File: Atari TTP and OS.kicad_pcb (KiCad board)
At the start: 2 copper layers, 19.6 x 52.1 mm, 13 parts, among them J1 Left, J2 Right, J4 Signals, J6 TTP_sel, U1 74LS157, U2 27C010, U3 74LVC2G74

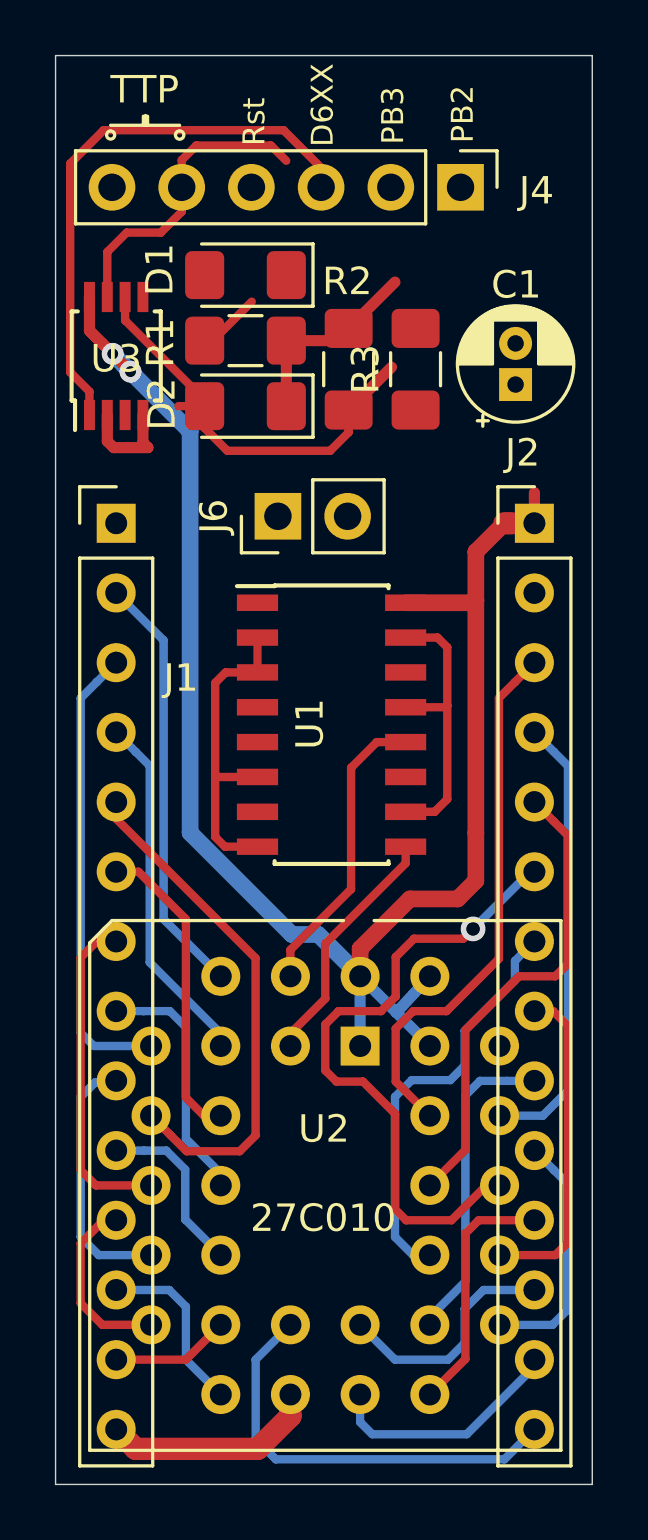
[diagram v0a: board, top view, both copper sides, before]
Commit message: Tracking
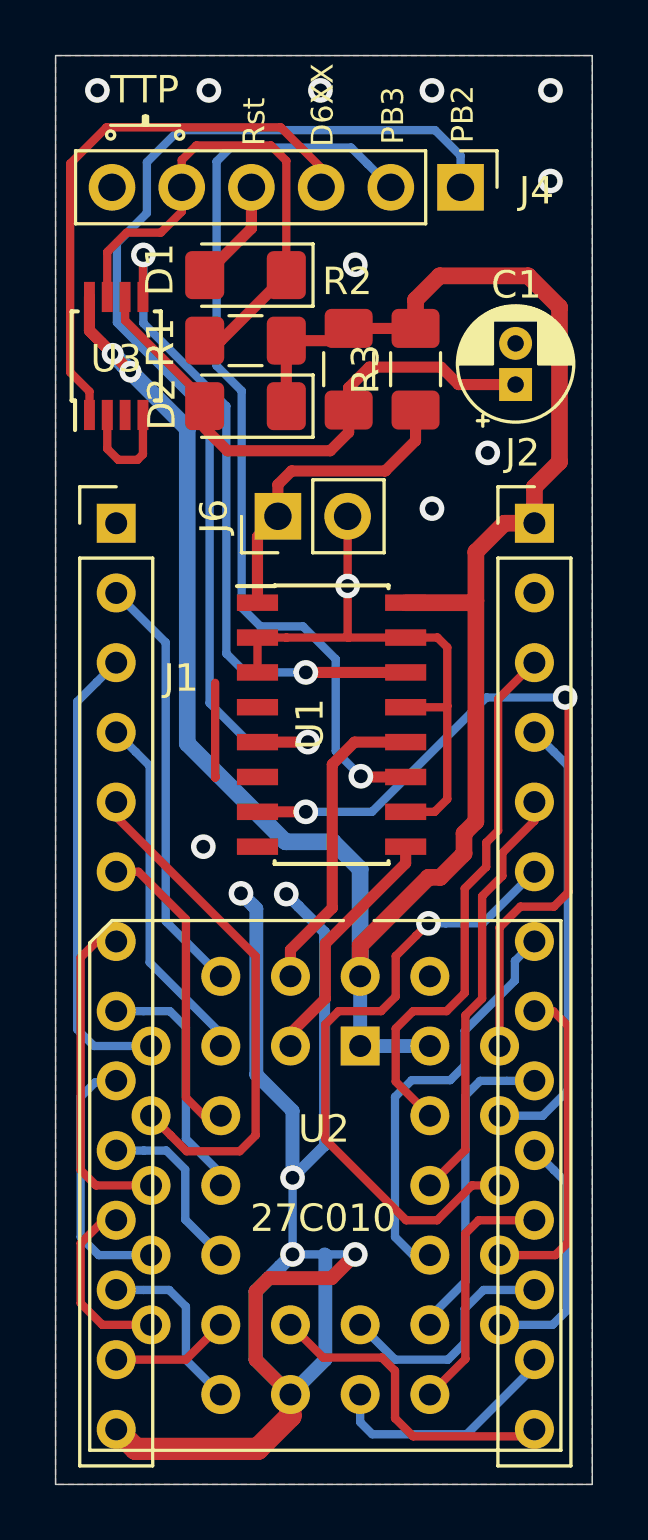
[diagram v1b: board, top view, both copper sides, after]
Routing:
- net GND: track 34.0 -> 85.1 mm, vias 0 -> 16
- net PB2: track 0.00 -> 41.0 mm, vias 0 -> 1
- net PB3: track 0.25 -> 34.5 mm, vias 0 -> 1
- net Net-(U1-Pad7): track 0.00 -> 27.4 mm, vias 0 -> 2
- net A16: track 0.00 -> 24.1 mm, vias 0 -> 2
- net VCC: track 69.4 -> 82.3 mm
- net Net-(J6-Pad1): track 0.00 -> 11.4 mm
- net Net-(D1-Pad1): track 13.4 -> 19.2 mm
- net Net-(C1-Pad1): track 16.5 -> 20.8 mm
- net D3: track 15.6 -> 11.7 mm
- net RST: track 0.63 -> 4.54 mm
- net A9: track 17.3 -> 15.5 mm
- net A11: track 23.6 -> 23.1 mm
- added copper zone on B.Cu, net GND
- added copper zone on F.Cu, net GND
